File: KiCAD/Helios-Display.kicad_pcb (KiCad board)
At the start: 2 copper layers, 3 parts, among them J1 Raspberry_Pi_2_3, J2 FFC_ST1633 (Touch), J3 Conn_01x45_Female

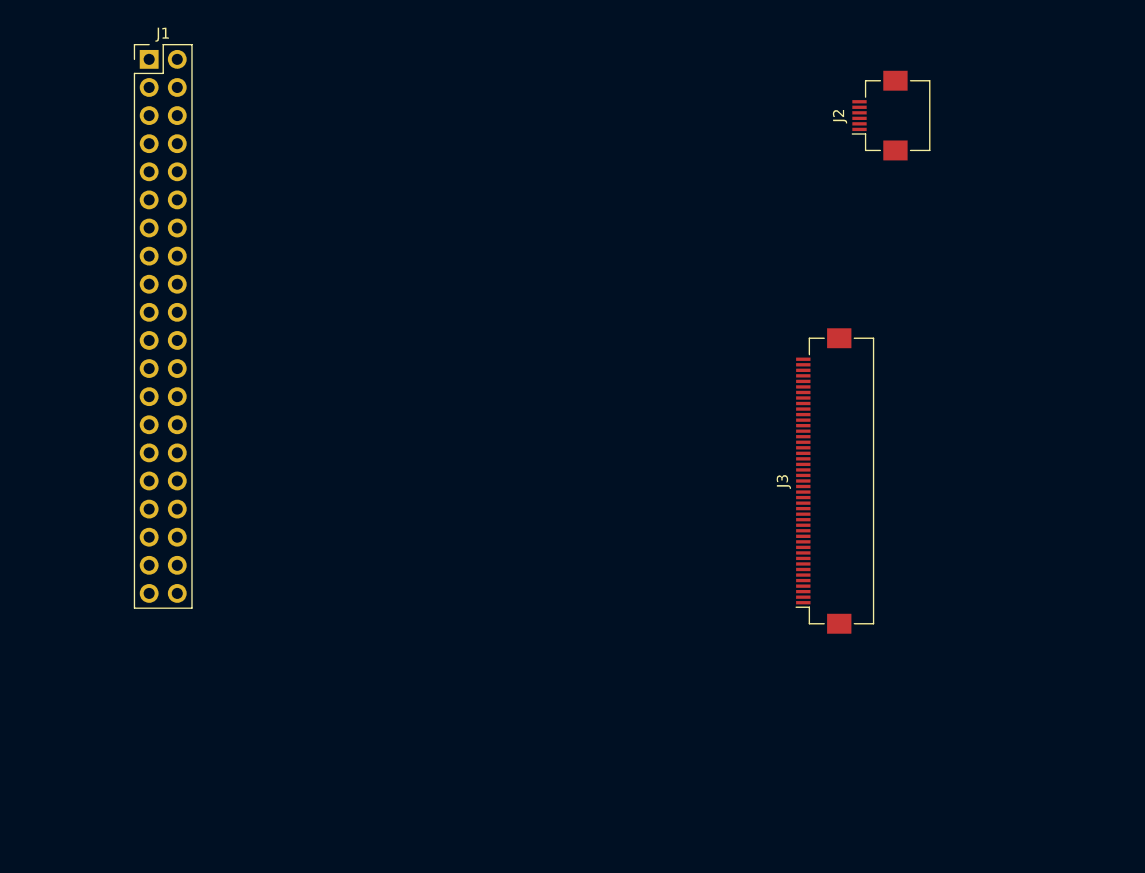
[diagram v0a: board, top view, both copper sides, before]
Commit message: updated KiCAD files
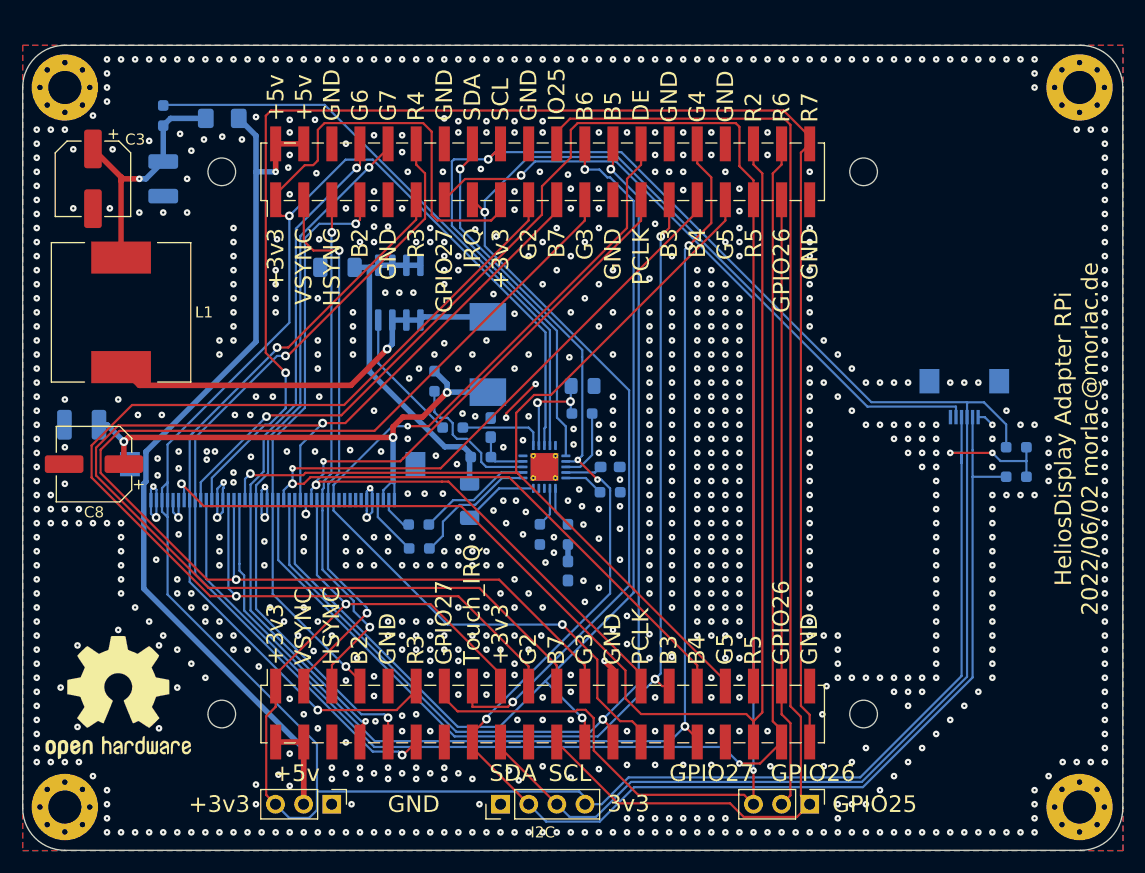
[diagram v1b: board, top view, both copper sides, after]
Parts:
- added C1: 470nF, Capacitor_SMD:C_0603_1608Metric_Pad1.08x0.95mm_HandSolder, B.Cu at (149.6, 119.9)
- added C2: 4.7uF/16V, Capacitor_SMD:C_1210_3225Metric_Pad1.33x2.70mm_HandSolder, B.Cu at (113.0, 84.5)
- added C3: 220uF/16V, Capacitor_SMD:CP_Elec_6.3x3, F.Cu at (106.7, 84.5)
- added C4: 0.47uF, Capacitor_SMD:C_0805_2012Metric_Pad1.18x1.45mm_HandSolder, B.Cu at (150.9, 103.2)
- added C5: 100nF, Capacitor_SMD:C_0603_1608Metric_Pad1.08x0.95mm_HandSolder, B.Cu at (153.4, 110.5)
- added C6: NC, Capacitor_SMD:C_0603_1608Metric_Pad1.08x0.95mm_HandSolder, B.Cu at (142.6, 106.9)
- added C7: 4.7uF/25V, Capacitor_SMD:C_1210_3225Metric_Pad1.33x2.70mm_HandSolder, B.Cu at (105.7, 106.7)
- added C8: 22uF/25V, Capacitor_SMD:CP_Elec_6.3x3, F.Cu at (106.8, 110.2)
- added D1: B360, Diode_SMD:D_SMC, B.Cu at (142.4, 100.3)
- added F1: Fuse, Fuse:Fuse_1206_3216Metric_Pad1.42x1.75mm_HandSolder, B.Cu at (118.4, 79.0)
- added H1: MountingHole_Pad, MountingHole:MountingHole_3mm_Pad_Via, F.Cu at (104.1, 141.2)
- added H2: MountingHole_Pad, MountingHole:MountingHole_3mm_Pad_Via, F.Cu at (195.8, 141.2)
- added H3: MountingHole_Pad, MountingHole:MountingHole_3mm_Pad_Via, F.Cu at (104.1, 76.2)
- added H4: MountingHole_Pad, MountingHole:MountingHole_3mm_Pad_Via, F.Cu at (195.8, 76.2)
- added H5: MountingHoleRaspi, MountingHole:MountingHole_2.5mm, F.Cu at (176.3, 83.8)
- added H6: MountingHoleRaspi, MountingHole:MountingHole_2.5mm, F.Cu at (118.3, 83.8)
- added H7: MountingHoleRaspi, MountingHole:MountingHole_2.5mm, F.Cu at (176.3, 132.8)
- added H8: MountingHoleRaspi, MountingHole:MountingHole_2.5mm, F.Cu at (118.3, 132.8)
- added J4: Power, Connector_PinHeader_2.54mm:PinHeader_1x03_P2.54mm_Vertical, F.Cu at (128.3, 141.0)
- added J6: I2C, Connector_PinHeader_2.54mm:PinHeader_1x04_P2.54mm_Vertical, F.Cu at (143.5, 141.0)
- added J7: GPIO, Connector_PinHeader_2.54mm:PinHeader_1x03_P2.54mm_Vertical, F.Cu at (171.4, 141.0)
- added J8: Raspberry_Pi_2_3, Connector_PinHeader_2.54mm:PinHeader_2x20_P2.54mm_Vertical_SMD, F.Cu at (147.3, 132.8)
- added L1: 33uH/3.5A, Inductor_SMD:L_12x12mm_H8mm, F.Cu at (109.2, 96.5)
- added M1: AM4490N, Package_SO:SOIC-8_3.9x4.9mm_P1.27mm, B.Cu at (134.4, 94.7)
- added OSHW_F: OSHW-Logo2_14.6x12mm_SilkScreen, Symbol:OSHW-Logo2_14.6x12mm_SilkScreen, F.Cu at (109.0, 131.3)
- added OSJW_B: OSHW-Logo2_14.6x12mm_SilkScreen, Symbol:OSHW-Logo2_14.6x12mm_SilkScreen, B.Cu at (109.0, 131.3)
- added R1: 270, Resistor_SMD:R_0603_1608Metric_Pad0.98x0.95mm_HandSolder, B.Cu at (149.6, 116.6)
- added R10: 0, Resistor_SMD:R_0603_1608Metric_Pad0.98x0.95mm_HandSolder, B.Cu at (141.7, 109.6)
- added R11: 50, Resistor_SMD:R_0603_1608Metric_Pad0.98x0.95mm_HandSolder, B.Cu at (190.1, 111.4)
- added R12: 50, Resistor_SMD:R_0603_1608Metric_Pad0.98x0.95mm_HandSolder, B.Cu at (190.1, 108.7)
- added R13: 0, Resistor_SMD:R_0603_1608Metric_Pad0.98x0.95mm_HandSolder, B.Cu at (136.1, 115.7)
- added R14: 0, Resistor_SMD:R_0603_1608Metric_Pad0.98x0.95mm_HandSolder, B.Cu at (136.2, 117.9)
- added R2: 100k, Resistor_SMD:R_0603_1608Metric_Pad0.98x0.95mm_HandSolder, B.Cu at (153.4, 112.8)
- added R3: R, Resistor_SMD:R_0603_1608Metric_Pad0.98x0.95mm_HandSolder, B.Cu at (147.1, 116.6)
- added R4: 100k, Resistor_SMD:R_0603_1608Metric_Pad0.98x0.95mm_HandSolder, B.Cu at (150.9, 105.7)
- added R5: 10, Resistor_SMD:R_0603_1608Metric_Pad0.98x0.95mm_HandSolder, B.Cu at (139.2, 106.9)
- added R6: 50m, Resistor_SMD:R_1206_3216Metric_Pad1.30x1.75mm_HandSolder, B.Cu at (128.8, 92.5)
- added R7: 0, Resistor_SMD:R_0603_1608Metric_Pad0.98x0.95mm_HandSolder, B.Cu at (113.0, 78.7)
- added R8: NC, Resistor_SMD:R_1206_3216Metric_Pad1.30x1.75mm_HandSolder, B.Cu at (140.7, 113.5)
- added R9: 0, Resistor_SMD:R_0603_1608Metric_Pad0.98x0.95mm_HandSolder, B.Cu at (137.5, 102.7)
- added U1: MP3385A, Package_DFN_QFN:QFN-20-1EP_4x4mm_P0.5mm_EP2.5x2.5mm_ThermalVias, B.Cu at (147.5, 110.5)
- J1: footprint Connector_PinHeader_2.54mm:PinHeader_2x20_P2.54mm_Vertical -> Connector_PinHeader_2.54mm:PinHeader_2x20_P2.54mm_Vertical_SMD
- J2: moved to B.Cu
- J3: value Conn_01x45_Female -> FFC_LCD; moved to B.Cu
- moved J3 49.8 mm to (122.9, 111.6), turned to 0 degrees
- moved J1 37.0 mm to (147.3, 83.8), turned to 90 degrees
- moved J2 26.5 mm to (185.4, 104.1), turned to 0 degrees
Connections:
- J1 pad 13: unconnected-(J1-Pad13) -> /GPIO27
- J1 pad 14: GNDPWR -> GNDA
- J1 pad 20: GNDPWR -> GNDA
- J1 pad 22: unconnected-(J1-Pad22) -> /GPIO25
- J1 pad 25: GNDPWR -> GNDA
- J1 pad 30: GNDPWR -> GNDA
- J1 pad 34: GNDPWR -> GNDA
- J1 pad 37: unconnected-(J1-Pad37) -> /GPIO26
- J1 pad 39: GNDPWR -> GNDA
- J1 pad 6: GNDPWR -> GNDA
- J1 pad 9: GNDPWR -> GNDA
- J2 pad 1: GNDPWR -> unconnected-(J2-Pad1)
- J2 pad 2: /GPIO_SDA -> /ST1633_IRQ
- J2 pad 3: /GPIO_SCL -> +3V3
- J2 pad 4: +3V3 -> /GPIO_SCL
- J2 pad 5: /ST1633_IRQ -> /GPIO_SDA
- J2 pad 6: unconnected-(J2-Pad6) -> GNDA
- J3 pad 1: GNDPWR -> GNDA
- J3 pad 13: /LCD_G_{0} -> GNDA
- J3 pad 14: /LCD_G_{1} -> GNDA
- J3 pad 2: GNDPWR -> GNDA
- J3 pad 21: /LCD_B_{0} -> GNDA
- J3 pad 22: /LCD_B_{1} -> GNDA
- J3 pad 29: GNDPWR -> GNDA
- J3 pad 31: /LCD_DISP -> +3V3
- J3 pad 40: GNDPWR -> GNDA
- J3 pad 41: GNDPWR -> GNDA
- J3 pad 45: /LCD_LED_A2 -> /LCD_LED_A1
- J3 pad 5: /LCD_R_{0} -> GNDA
- J3 pad 6: /LCD_R_{1} -> GNDA
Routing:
- net +3V3: track 0.00 -> 300.7 mm, vias 0 -> 4
- net /GPIO_SCL: track 0.00 -> 170.7 mm, vias 0 -> 1
- net /GPIO_SDA: track 0.00 -> 146.9 mm, vias 0 -> 4
- net /LCD_R_{7}: track 0.00 -> 144.2 mm, vias 0 -> 1
- net /LCD_R_{6}: track 0.00 -> 121.5 mm, vias 0 -> 1
- net /LCD_R_{2}: track 0.00 -> 118.3 mm, vias 0 -> 1
- net /LCD_R_{5}: track 0.00 -> 117.9 mm, vias 0 -> 1
- net /ST1633_IRQ: track 0.00 -> 116.9 mm, vias 0 -> 2
- net /LCD_G_{3}: track 0.00 -> 116.4 mm, vias 0 -> 1
- net /GPIO27: track 0.00 -> 115.0 mm, vias 0 -> 2
- net /LCD_B_{7}: track 0.00 -> 112.5 mm, vias 0 -> 1
- net /LCD_G_{4}: track 0.00 -> 111.5 mm, vias 0 -> 2
- net /GPIO25: track 0.00 -> 111.2 mm
- net /LCD_G_{2}: track 0.00 -> 110.0 mm, vias 0 -> 1
- net /LCD_B_{6}: track 0.00 -> 97.8 mm, vias 0 -> 2
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- added copper zone on B.Cu, net GNDA
- added copper zone on F.Cu, net GNDA
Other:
- board outline added: 99.4 x 72.7 mm
- board text added: "+3v3"
- board text added: "+5v"
- board text added: "3v3"
- board text added: "B2"
- board text added: "B3"
- board text added: "B4"
- board text added: "B5"
- board text added: "B6"
- board text added: "B7"
- board text added: "DE"
- board text added: "G2"
- board text added: "G3"
- board text added: "G4"
- board text added: "G5"
- board text added: "G6"
- board text added: "G7"
- board text added: "GND"
- board text added: "GPIO25"
- board text added: "GPIO26"
- board text added: "GPIO27"
- board text added: "HSYNC"
- board text added: "HeliosDisplay Adapter RPi 2022/06/02 morlac@morlac.de"
- board text added: "IO25"
- board text added: "IRQ"
- board text added: "PCLK"
- board text added: "R2"
- board text added: "R3"
- board text added: "R4"
- board text added: "R5"
- board text added: "R6"
- board text added: "R7"
- board text added: "SCL"
- board text added: "SDA"
- board text added: "Touch_IRQ"
- board text added: "VSYNC"
